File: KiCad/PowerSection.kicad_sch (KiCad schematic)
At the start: 24 parts, among them U2 LM7805_TO220, U4 LM337_TO220, U6 MC34063AP, U7 LM7810_TO220

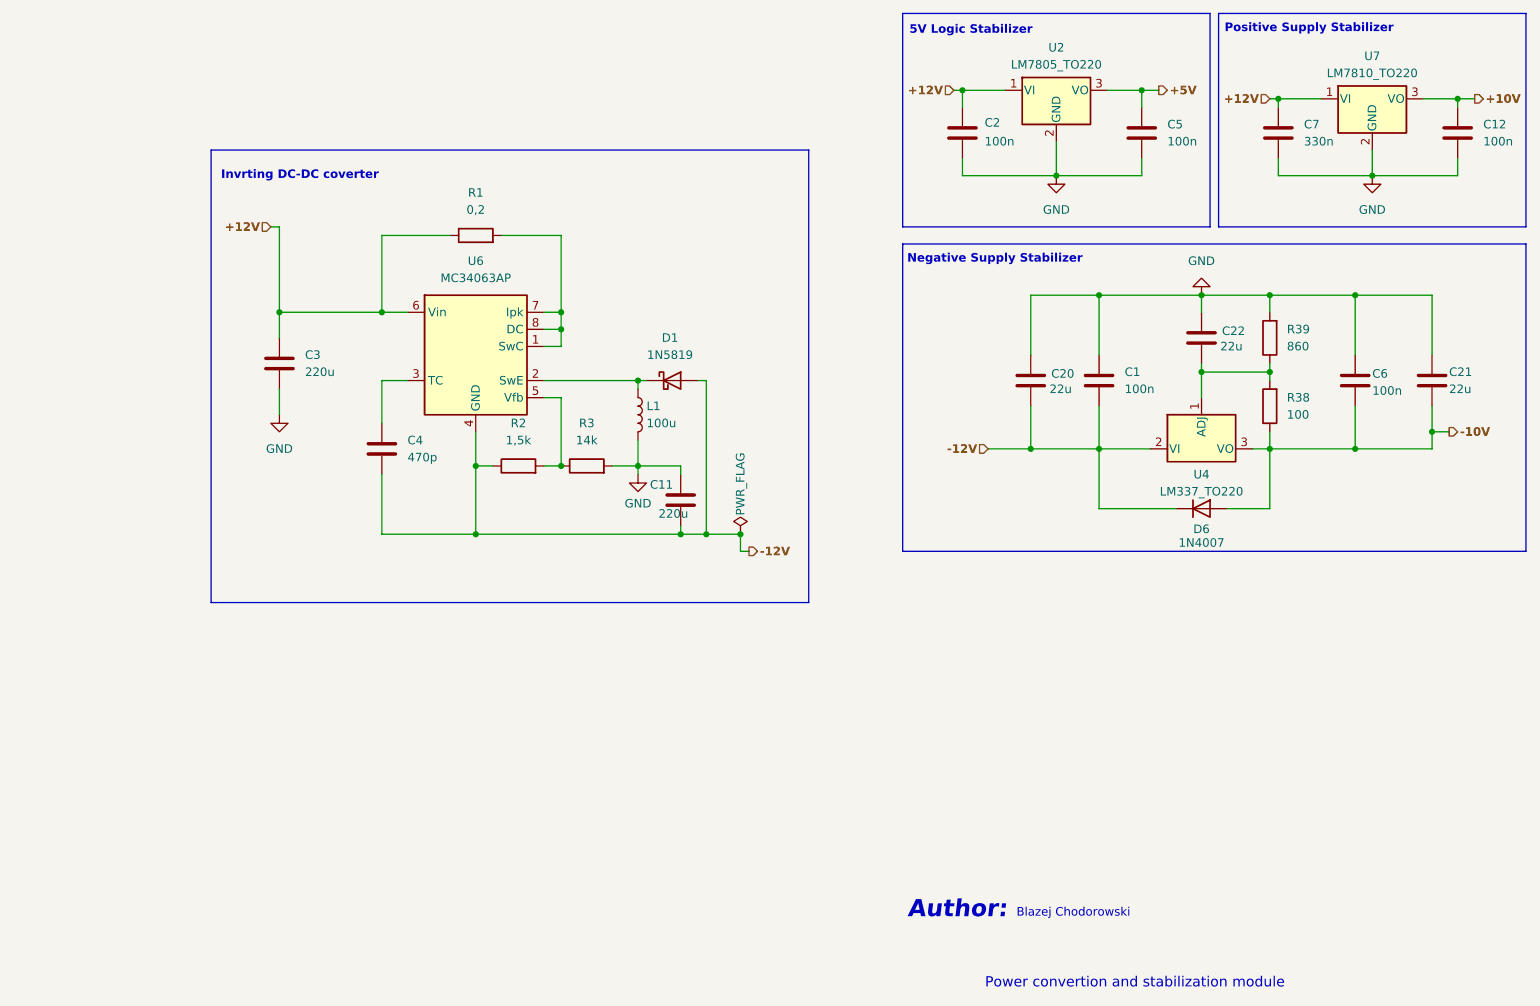
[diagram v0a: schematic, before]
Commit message: minor changes
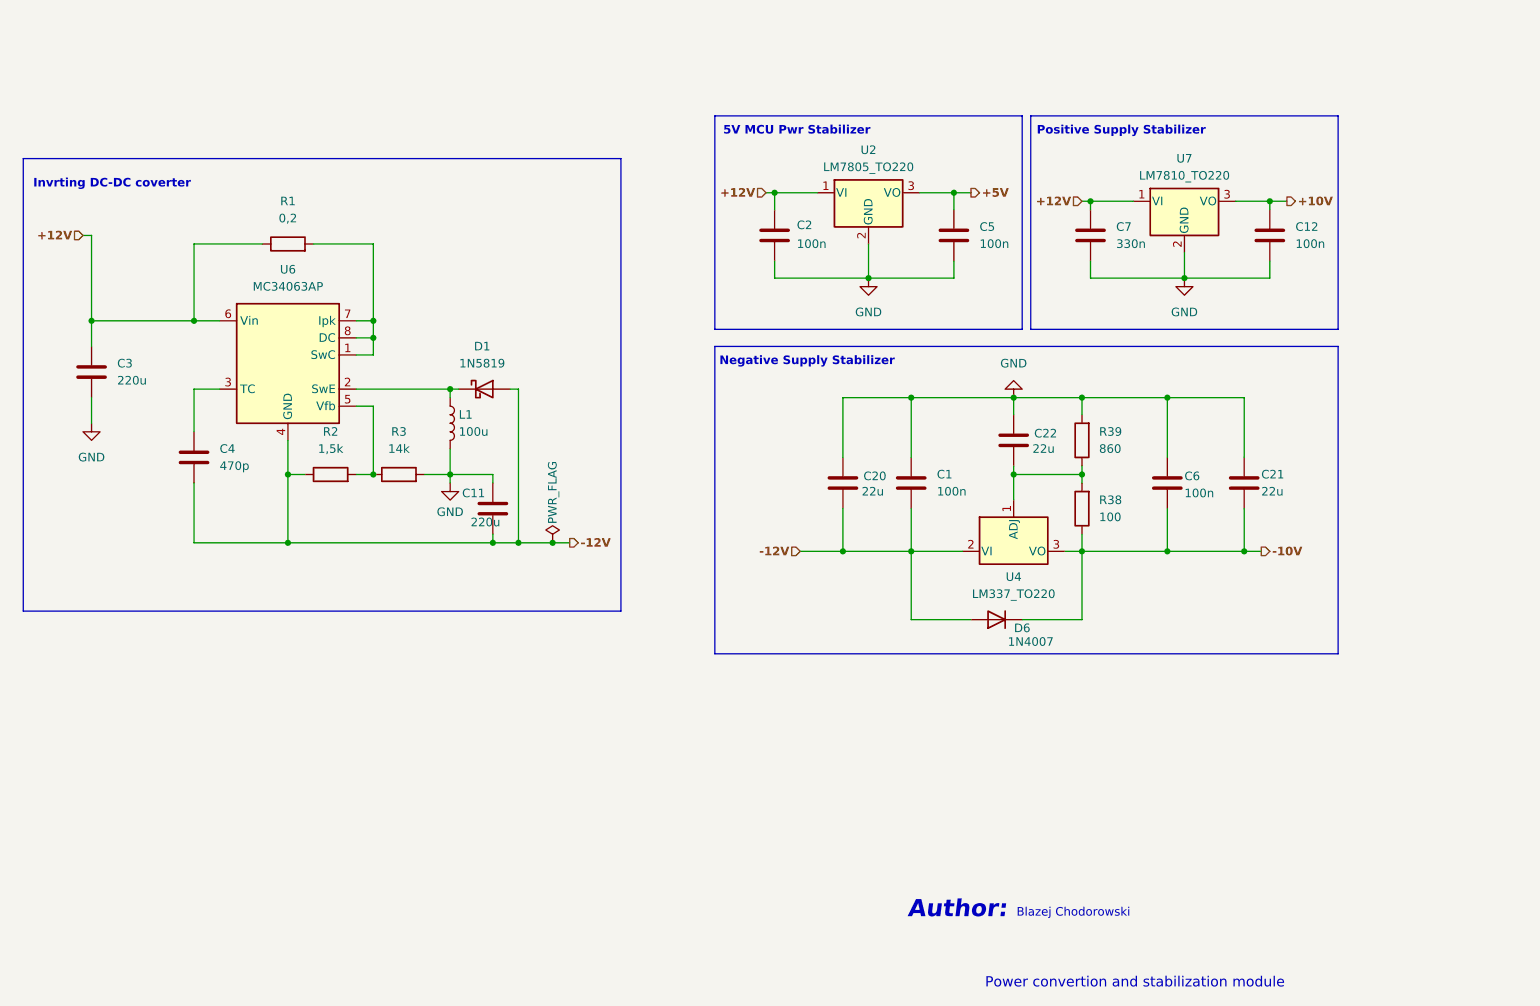
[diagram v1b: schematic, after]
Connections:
- net -10V: now also D6.1 (K); no longer D6.2 (A)
- net -12V: now also D6.2 (A); no longer D6.1 (K)
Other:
- note added: "5V MCU Pwr Stabilizer"
- note removed: "5V Logic Stabilizer"
- moved on the sheet: C1, C11, C12, C2, C20, C21, C22, C3, C4, C5, C6, C7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
